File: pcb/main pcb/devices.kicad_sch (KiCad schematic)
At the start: 33 parts, among them J3 Conn_01x03, Q1 AO3401A, SW2 JS102011JCQN, SW4 SW_DIP_x02, U10 SHT31-DIS, U3 LIS3DH, U5 TP4057, U6 XC6206P332MR

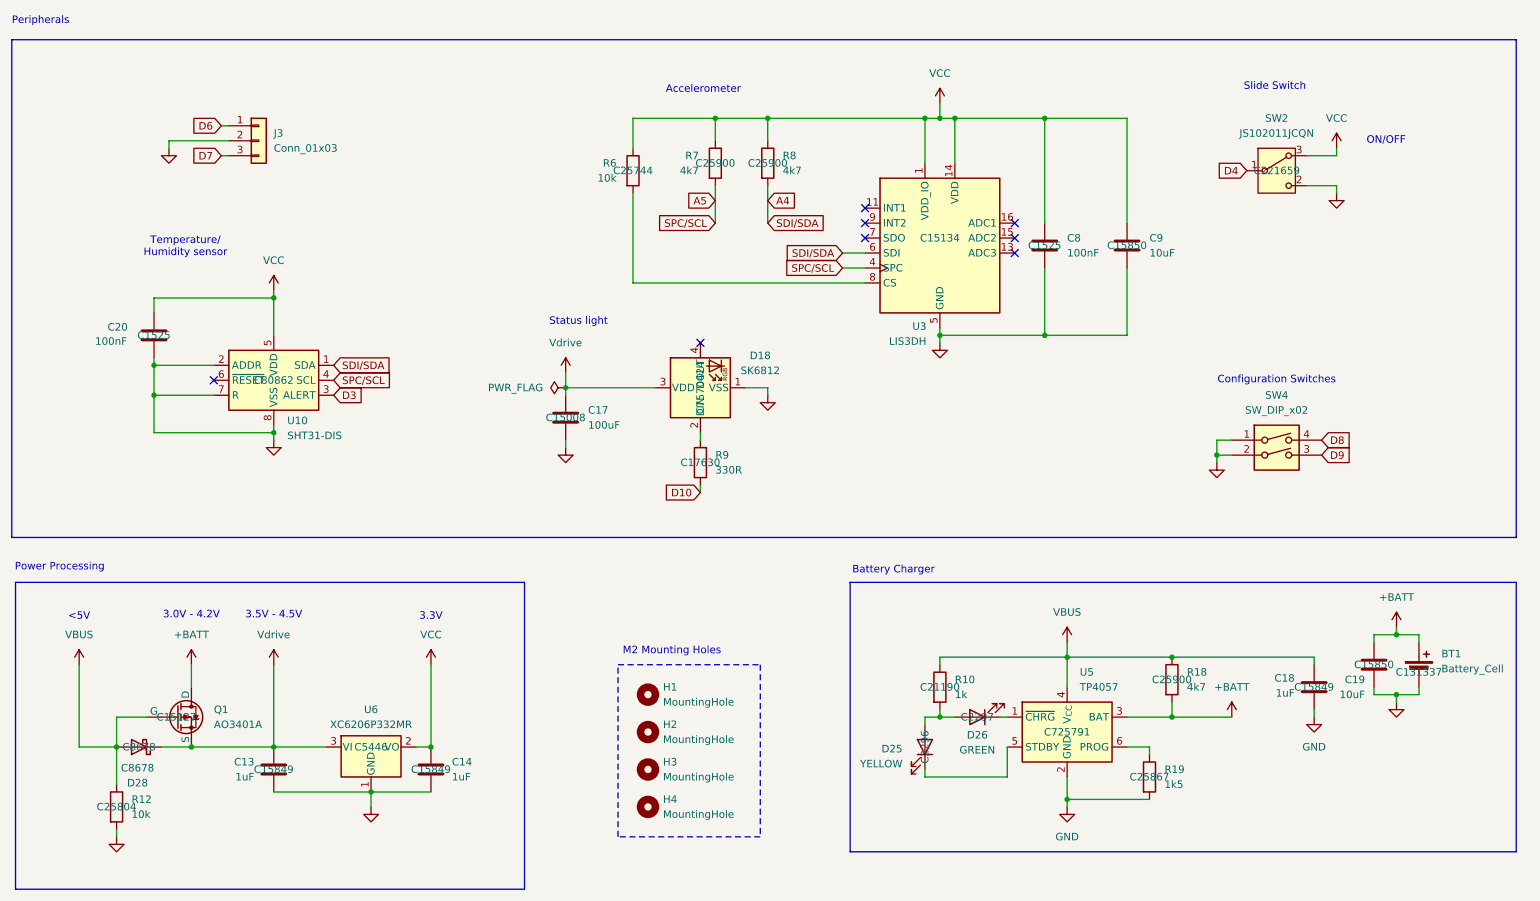
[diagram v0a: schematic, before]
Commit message: fixed pcb
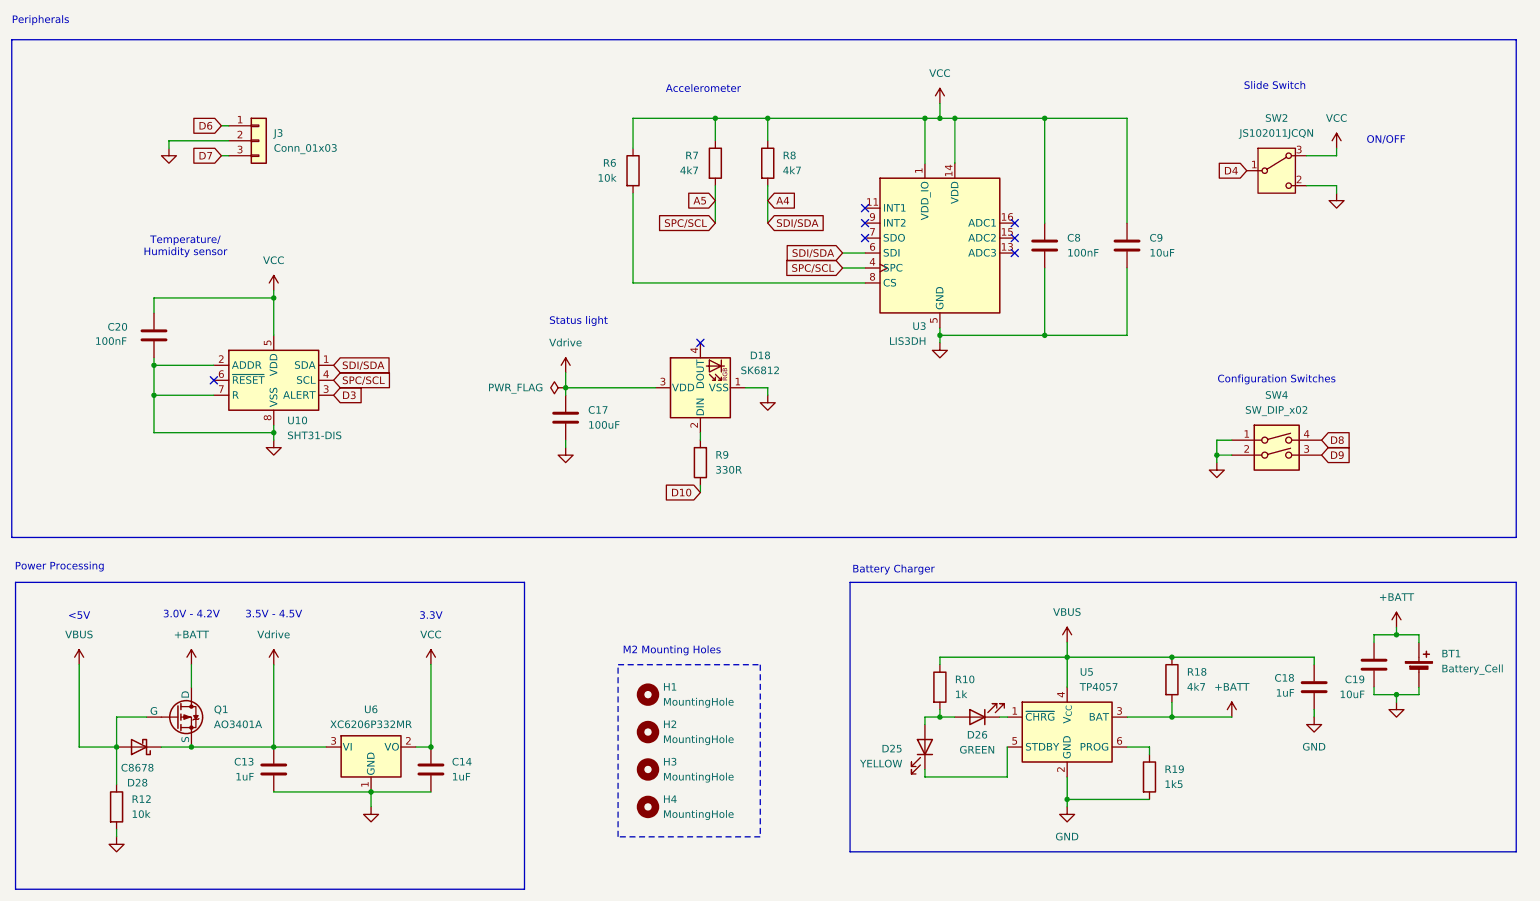
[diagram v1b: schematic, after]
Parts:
- BT1: LCSC C131337 -> (none)
- C13, C14, C18: LCSC C15849 -> (none)
- C17: LCSC C15008 -> (none)
- C19, C9: LCSC C15850 -> (none)
- C20, C8: LCSC C1525 -> (none)
- D18: LCSC C7570424 -> (none)
- D25: LCSC C2296 -> (none)
- D26: LCSC C2297 -> (none)
- D28: LCSC C8678 -> (none)
- Q1: LCSC C15127 -> (none)
- R10: LCSC C21190 -> (none)
- R12: LCSC C25804 -> (none)
- R18, R7, R8: LCSC C25900 -> (none)
- R19: LCSC C25867 -> (none)
- R6: LCSC C25744 -> (none)
- R9: LCSC C17630 -> (none)
- SW2: LCSC C221659 -> (none)
- U10: LCSC C80862 -> (none)
- U3: LCSC C15134 -> (none)
- U5: LCSC C725791 -> (none)
- U6: LCSC C5446 -> (none)
